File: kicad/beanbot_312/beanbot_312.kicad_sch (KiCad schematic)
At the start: 45 parts, among them M1 P&O2_MEETPUNT, M10 P&O2_RGB_LED, M11 P&O2_RESISTOR, M12 P&O2_MEETPUNT, M13 P&O2_RESISTOR, M14 P&O2_MOSFET, M15 P&O2_RESISTOR, M16 P&O2_ULTRASONE_HC_SR04, M17 P&O2_MEETPUNT, M18 P&O2_MEETPUNT, M19 P&O2_MEETPUNT, M2 P&O2_MEETPUNT, M20 P&O2_MEETPUNT, M21 P&O2_GEWICHTSENSOR2, M23 P&O2_MEETPUNT, M24 P&O2_MEETPUNT, M25 P&O2_KLEURSENSOR, M26 P&O2_MEETPUNT, M27 P&O2_MEETPUNT, M28 P&O2_MEETPUNT, M29 P&O2_RELAIS-DP, M3 P&O2_RESISTOR, M30 P&O2_DC-MOTOR, M31 P&O2_RELAIS-DP, M32 P&O2_DC-MOTOR, M35 P&O2_DIODE, M36 P&O2_DIODE, M38 P&O2_MEETPUNT, M39 P&O2_MEETPUNT, M4 P&O2_MOSFET, M41 P&O2_MEETPUNT, M42 P&O2_MEETPUNT, M44 P&O2_RESISTOR, M45 P&O2_RESISTOR, M47 P&O2_MOSFET, M48 P&O2_MOSFET, M5 P&O2_RESISTOR, M50 P&O2_MEETPUNT, M51 P&O2_MEETPUNT, M6 P&O2_MEETPUNT, M7 P&O2_RESISTOR, M8 P&O2_MOSFET, M9 P&O2_RESISTOR, U1 P&O2_ARDUINO_MEGA_SHIELD

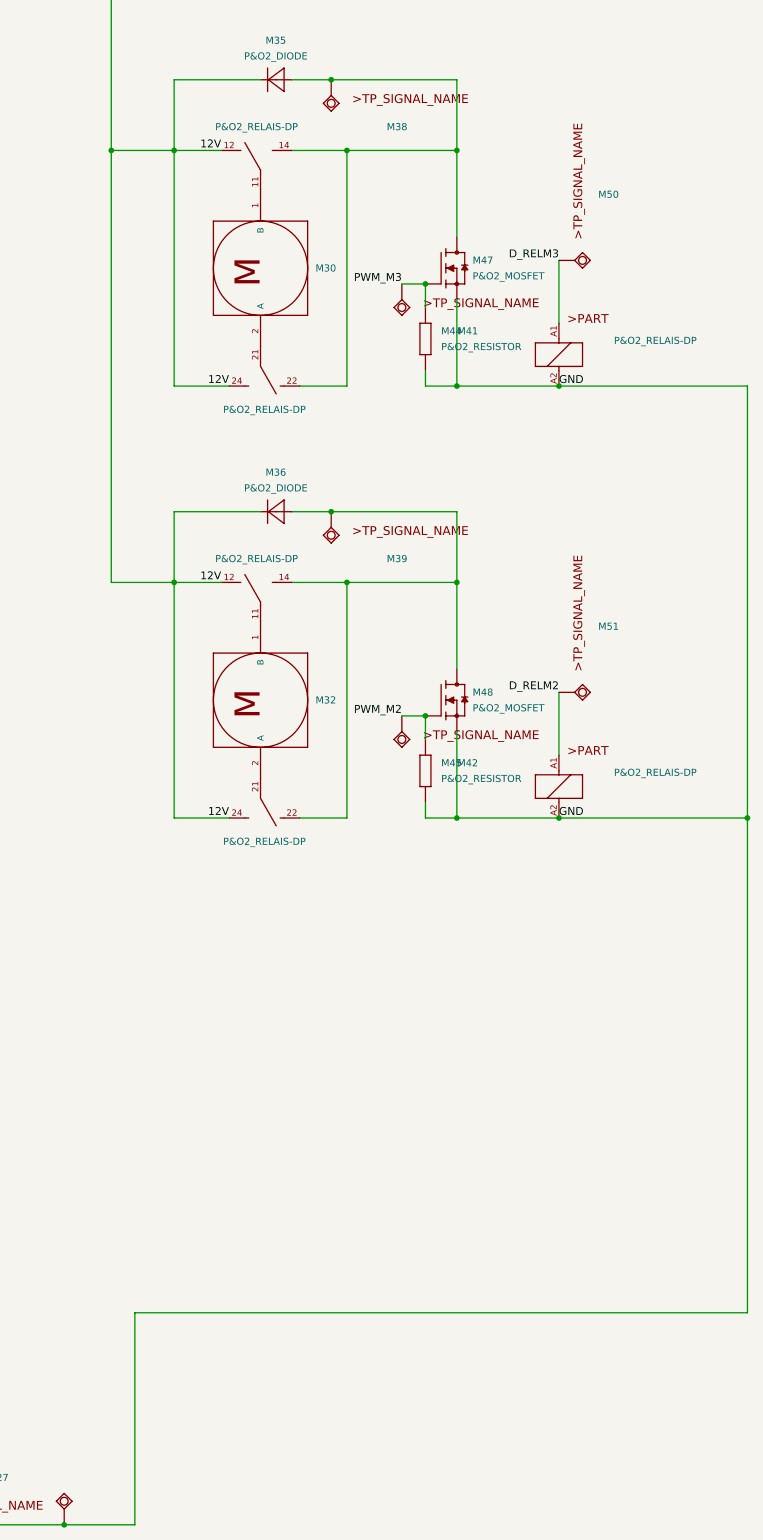
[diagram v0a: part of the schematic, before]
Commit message: Backups
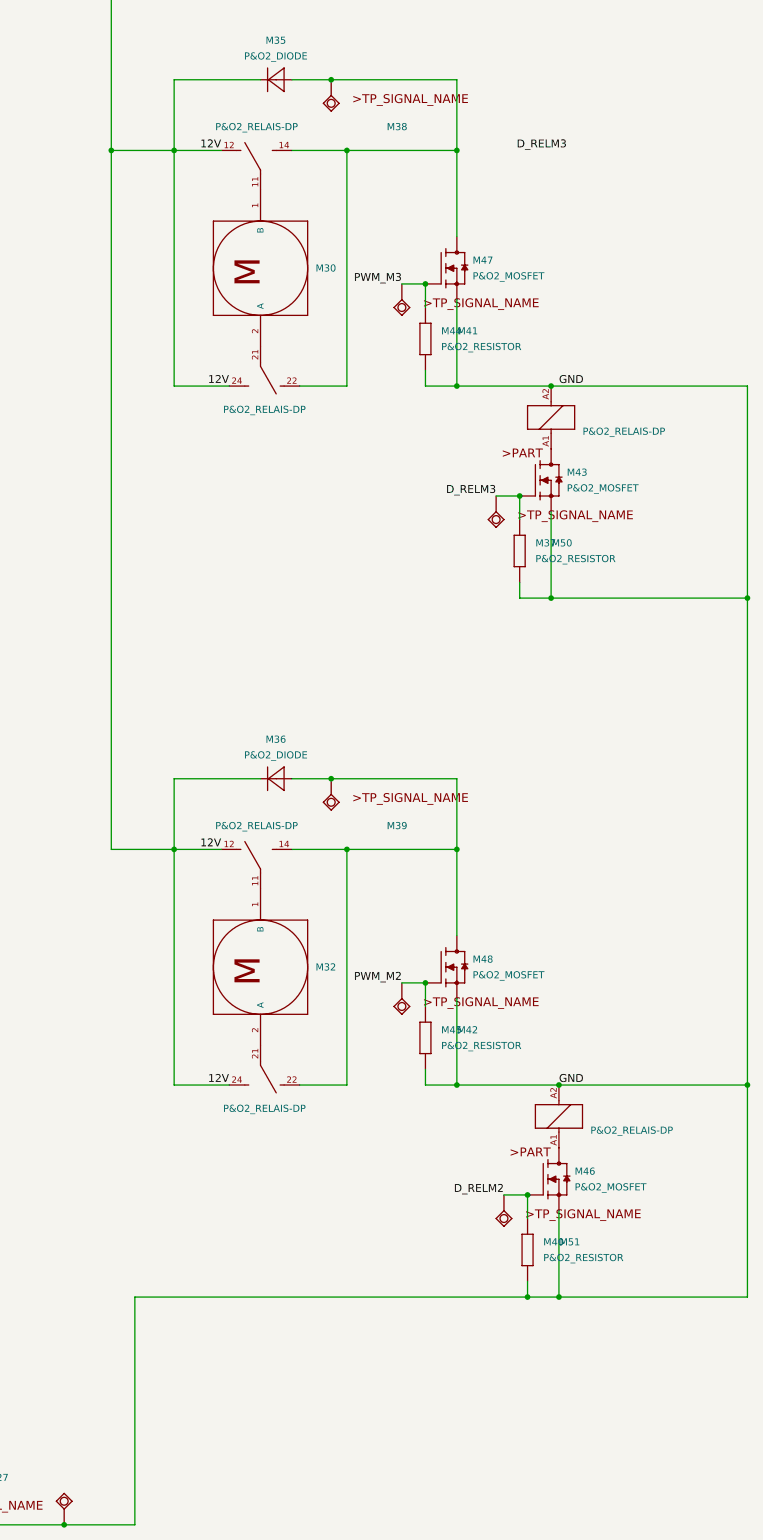
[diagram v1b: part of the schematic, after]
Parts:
- added M37, M40: P&O2_RESISTOR, 1_P&O2_lib:P&O2_RESISTOR, symbol 1_P&O2_lib:P&O2_RESISTOR
- added M43, M46: P&O2_MOSFET, 1_P&O2_lib:P&O2_TO220, symbol 1_P&O2_lib:P&O2_MOSFET
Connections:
- net D_RELM2: now also M40.1, M46.1 (eG); no longer M31.A1 (1)
- net D_RELM3: now also M37.1, M43.1 (eG); no longer M29.A1 (1)
- net GND: now also M37.2, M40.2, M43.3 (S), M46.3 (S)
- new net: M31.A1 (1), M46.2 (D)
- new net: M29.A1 (1), M43.2 (D)
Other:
- moved on the sheet: M32, M36, M39, M42, M45, M48, M50, M51
